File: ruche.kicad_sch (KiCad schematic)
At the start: 36 parts, among them IC2 MAX17048G+, IC3 L86-M33, IC4 SHT41-AD1B-R3, J13 Micro_SD_Card, U1 MKRWAN_1310, U2 MS5611-01BA, U3 XC6220B331MR

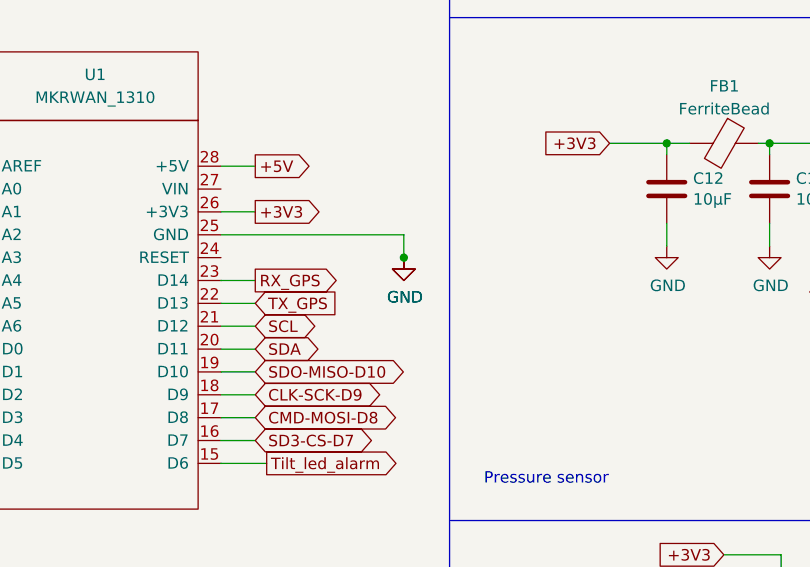
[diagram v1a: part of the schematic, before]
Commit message: update
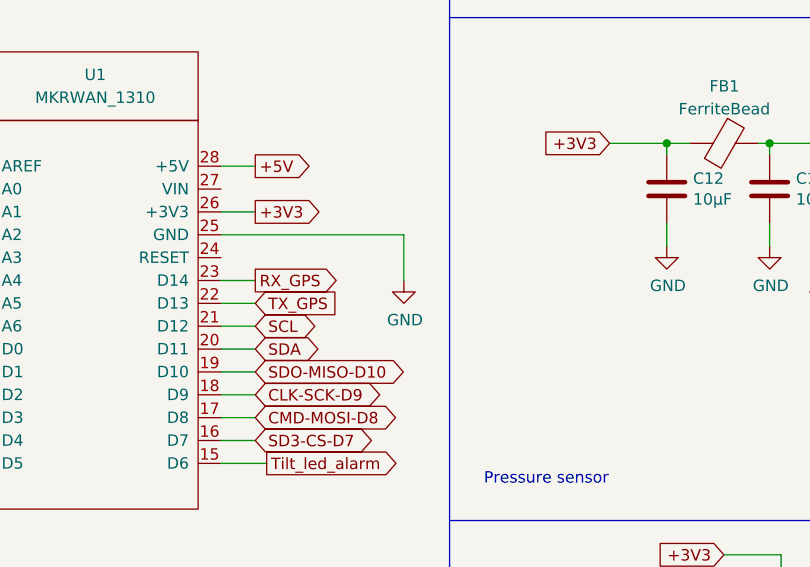
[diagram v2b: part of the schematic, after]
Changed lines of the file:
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@@
   (junction (at 53.34 72.39) (diameter 0) (color 0 0 0 0)
   )
-  (junction (at 191.77 91.44) (diameter 0) (color 0 0 0 0)
-  )
   (junction (at 220.98 78.74) (diameter 0) (color 0 0 0 0)
   )
@@
     (stroke (width 0) (type default) (color 0 0 0 0))
   )
+  (wire (pts (xy 191.77 88.9) (xy 191.77 93.98))
+    (stroke (width 0) (type default) (color 0 0 0 0))
+  )
   (wire (pts (xy 113.03 96.52) (xy 118.11 96.52))
     (stroke (width 0) (type default) (color 0 0 0 0))
@@
   )
   (wire (pts (xy 30.48 88.9) (xy 68.58 88.9))
-    (stroke (width 0) (type default) (color 0 0 0 0))
-  )
-  (wire (pts (xy 191.77 88.9) (xy 191.77 91.44))
     (stroke (width 0) (type default) (color 0 0 0 0))
   )
@@
     (pin "1")
   )
-  (symbol (lib_id "power:GND") (at 191.77 91.44 0) (unit 1)
-    (in_bom yes) (on_board yes)
-    (property "Reference" "#PWR0124" (id 0) (at 191.77 97.79 0)
-      (effects (font (size 1.27 1.27)) hide)
-    )
-    (property "Value" "GND" (id 1) (at 191.897 95.8342 0))
-    (property "Footprint" "" (id 2) (at 191.77 91.44 0)
-      (effects (font (size 1.27 1.27)) hide)
-    )
-    (property "Datasheet" "" (id 3) (at 191.77 91.44 0)
-      (effects (font (size 1.27 1.27)) hide)
-    )
-    (pin "1")
-  )
-  (symbol (lib_id "power:GND") (at 191.77 91.44 0) (unit 1)
-    (in_bom yes) (on_board yes)
-    (property "Reference" "#PWR0125" (id 0) (at 191.77 97.79 0)
-      (effects (font (size 1.27 1.27)) hide)
-    )
-    (property "Value" "GND" (id 1) (at 191.897 95.8342 0))
-    (property "Footprint" "" (id 2) (at 191.77 91.44 0)
-      (effects (font (size 1.27 1.27)) hide)
-    )
-    (property "Datasheet" "" (id 3) (at 191.77 91.44 0)
+  (symbol (lib_id "power:GND") (at 191.77 93.98 0) (unit 1)
+    (in_bom yes) (on_board yes)
+    (property "Reference" "#PWR0125" (id 0) (at 191.77 100.33 0)
+      (effects (font (size 1.27 1.27)) hide)
+    )
+    (property "Value" "GND" (id 1) (at 191.897 98.3742 0))
+    (property "Footprint" "" (id 2) (at 191.77 93.98 0)
+      (effects (font (size 1.27 1.27)) hide)
+    )
+    (property "Datasheet" "" (id 3) (at 191.77 93.98 0)
       (effects (font (size 1.27 1.27)) hide)
     )
@@
       (reference "#PWR0123") (unit 1) (value "GND") (footprint "")
     )
-    (path "/00000000-0000-0000-0000-000062832503"
-      (reference "#PWR0124") (unit 1) (value "GND") (footprint "")
-    )
     (path "/00000000-0000-0000-0000-000062832ae7"

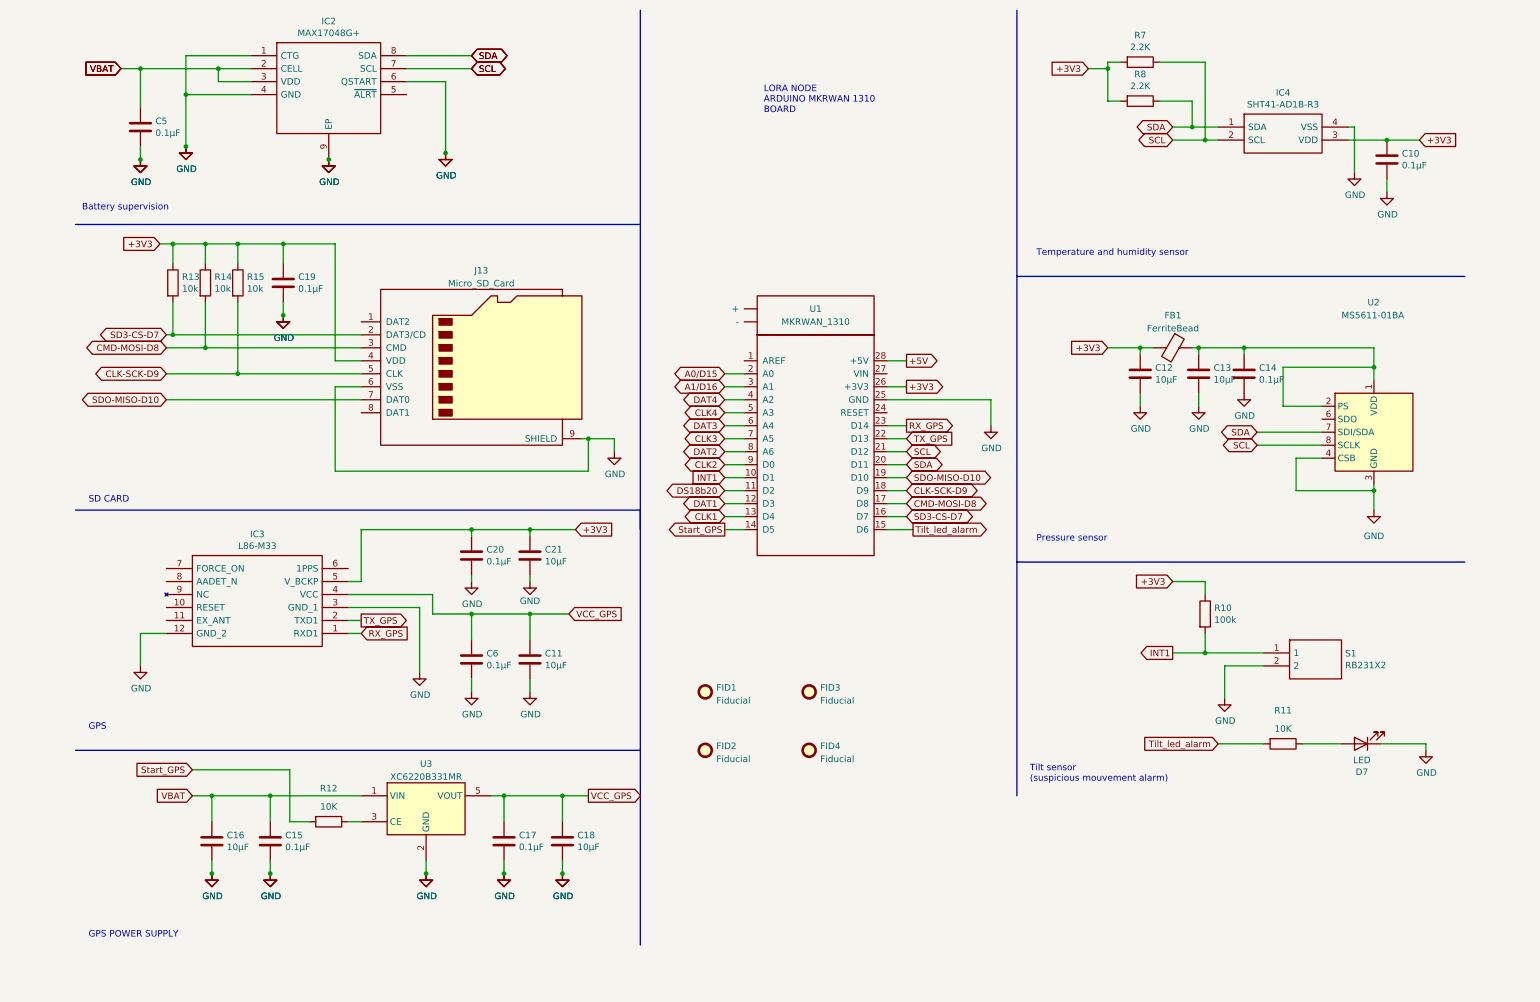
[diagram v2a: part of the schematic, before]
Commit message: Update
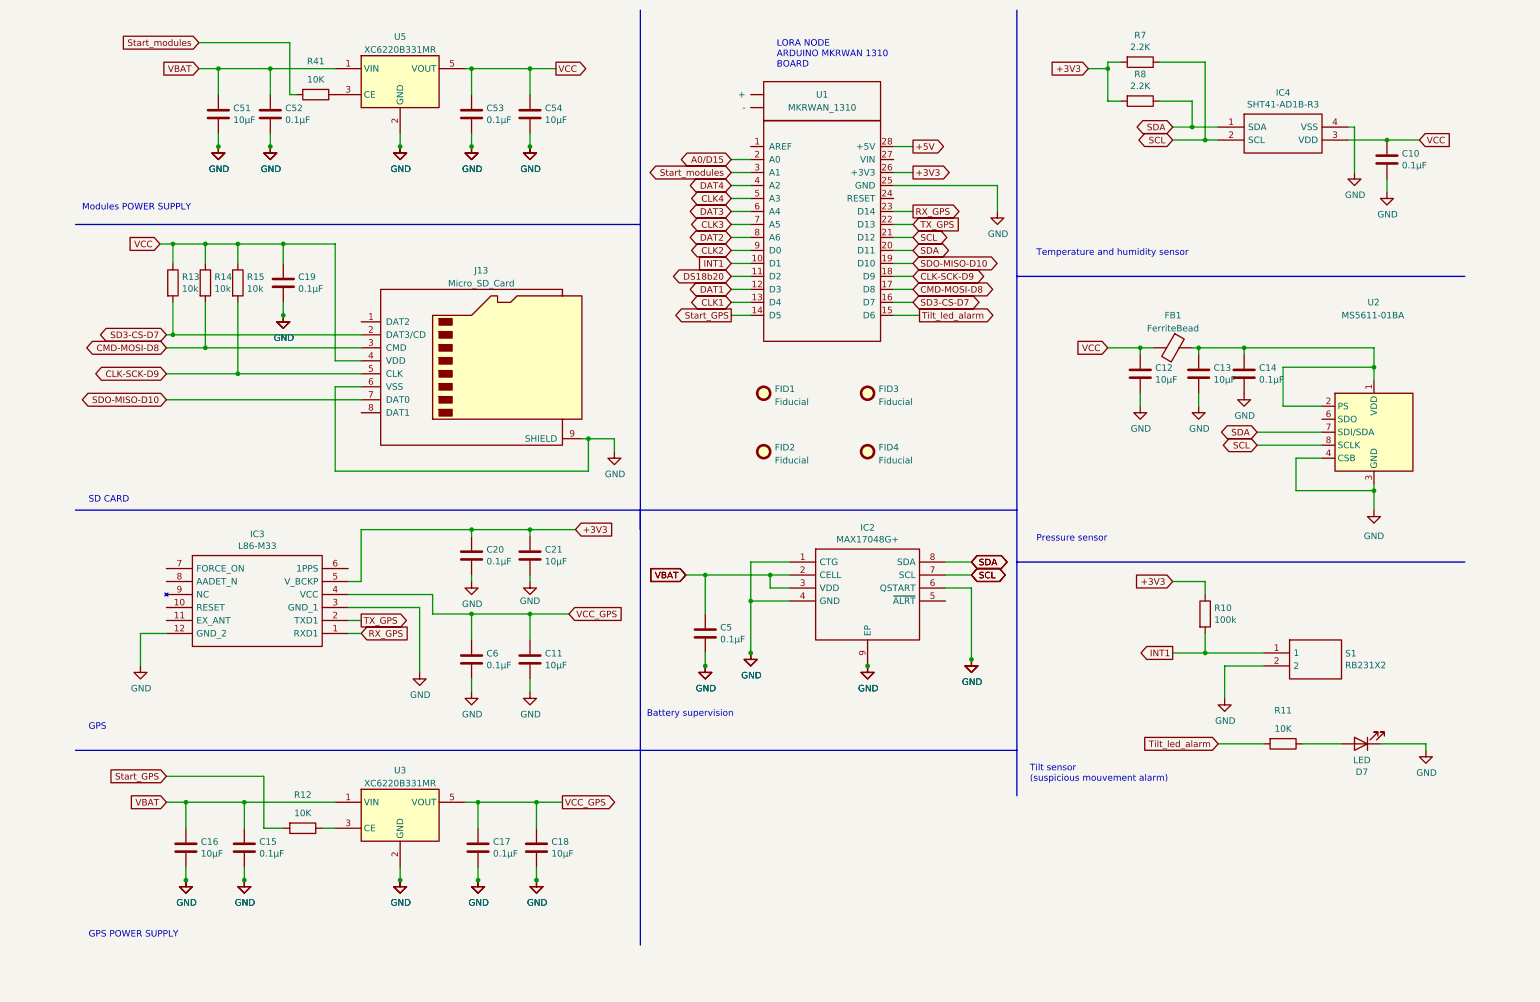
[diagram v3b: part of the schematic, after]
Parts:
- added C51: 10µF, Capacitor_SMD:C_0603_1608Metric, symbol Device:C
- added C52: 0.1µF, Capacitor_SMD:C_0805_2012Metric, symbol Device:C
- added C53: 0.1µF, Capacitor_SMD:C_0603_1608Metric, symbol Device:C
- added C54: 10µF, Capacitor_SMD:C_0805_2012Metric, symbol Device:C
- added R41: 10K, Resistor_SMD:R_0603_1608Metric, symbol Device:R
- added U5: XC6220B331MR, Package_TO_SOT_SMD:SOT-23-5, symbol Regulator_Linear:XC6220B331MR
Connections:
- net +3V3: no longer C10.1, C12.1, C19.1, FB1.2, IC4.3 (VDD), J13.4 (VDD), R13.1, R14.1, R15.1
- net GND: now also C51.2, C52.2, C53.2, C54.2, U5.2 (GND)
- net VBAT: now also C51.1, C52.1, U5.1 (VIN)
- net A1/D16 renamed Start_modules
- net Start_modules: now also R41.2
- new net: R41.1, U5.3 (CE)
- new net VCC: C10.1, C12.1, C19.1, C53.1, C54.1, FB1.2, IC4.3 (VDD), J13.4 (VDD), R13.1, R14.1, R15.1, U5.5 (VOUT)
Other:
- note added: "Modules POWER SUPPLY"
- moved on the sheet: C15, C16, C17, C18, C5, FID1, FID2, FID3, FID4, IC2, R12, U1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
